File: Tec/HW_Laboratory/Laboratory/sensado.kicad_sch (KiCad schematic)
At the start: 3 parts, among them U5 INA3221, U6 INA3221, U7 LM75B

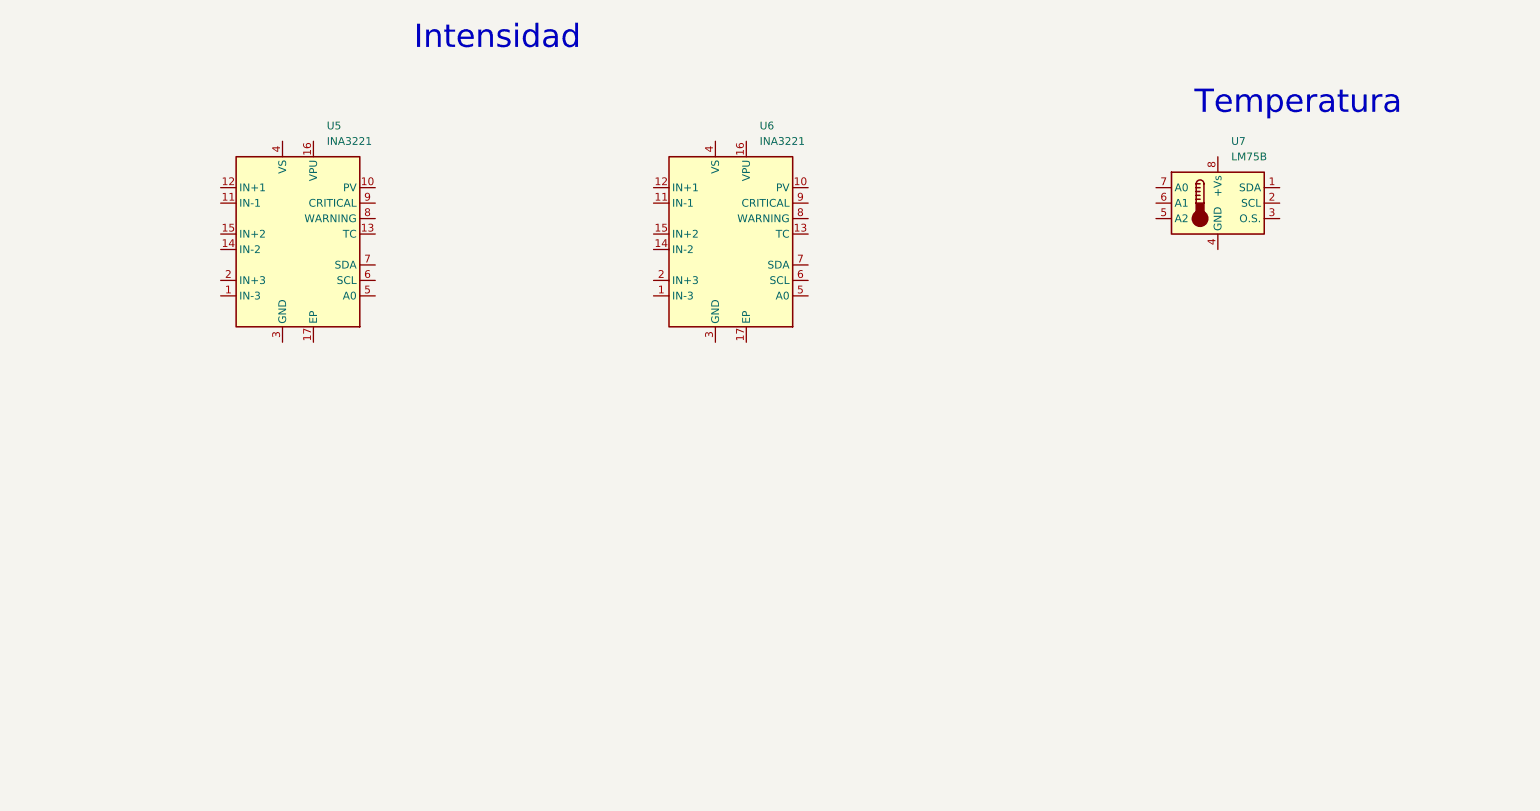
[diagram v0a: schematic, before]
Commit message: Schematics UPDATE
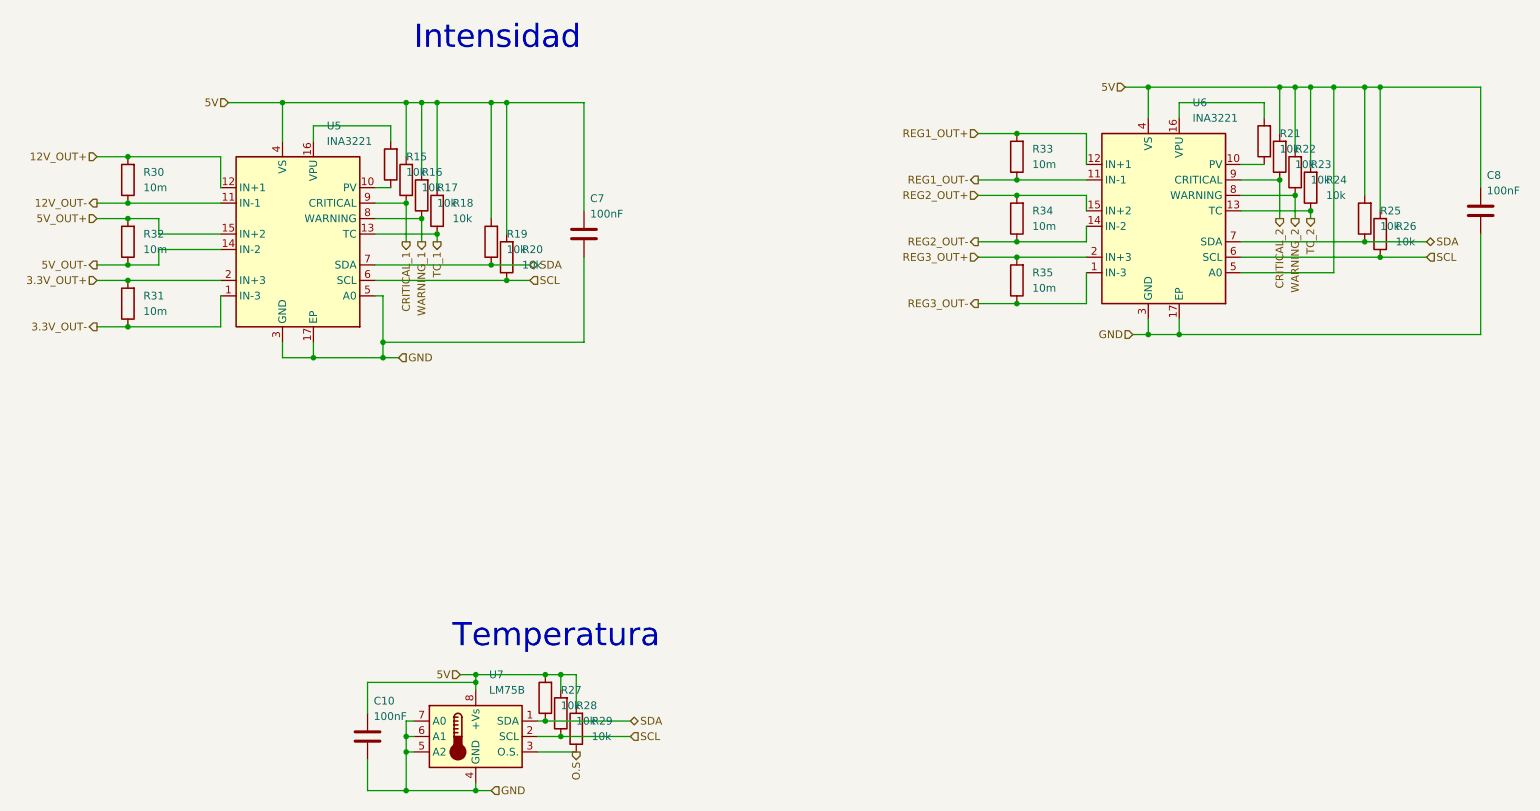
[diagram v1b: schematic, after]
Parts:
- added C10, C7, C8: 100nF, Capacitor_SMD:C_0603_1608Metric, symbol Device:C
- added R15, R16, R17, R18, R19, R20, R21, R22, R23, R24, R25, R26, R27, R28, R29: 10k, Resistor_SMD:R_0603_1608Metric, symbol Device:R
- added R30, R31, R32, R33, R34, R35: 10m, Resistor_SMD:R_2512_6332Metric, symbol Device:R
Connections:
- net 3.3V_OUT-: now reaches U5.1 (IN-3)
- net 3.3V_OUT-: now also R31.1
- net at U5.10 (PV): now also R15.1
- net 12V_OUT-: now reaches U5.11 (IN-1)
- net 12V_OUT-: now also R30.1
- net 12V_OUT+: now reaches U5.12 (IN+1)
- net 12V_OUT+: now also R30.2
- net TC_1: now reaches U5.13 (TC)
- net TC_1: now also R18.1
- net 5V_OUT-: now reaches U5.14 (IN-2)
- net 5V_OUT-: now also R32.1
- net 5V_OUT+: now reaches U5.15 (IN+2)
- net 5V_OUT+: now also R32.2
- net at U5.16 (VPU): now also R15.2
- net GND: now reaches U5.17 (EP)
- net GND: now also U5.3 (GND), U5.5 (A0), U6.17 (EP), U6.3 (GND), U7.4 (GND), U7.5 (A2), U7.6 (A1), U7.7 (A0), C10.2, C7.2, C8.2
- net 3.3V_OUT+: now reaches U5.2 (IN+3)
- net 3.3V_OUT+: now also R31.2
- net 5V: now reaches U5.4 (VS)
- net 5V: now also U6.4 (VS), U6.5 (A0), U7.8 (+Vs), C10.1, C7.1, C8.1, R16.2, R17.2, R18.2, R19.2, R20.2, R22.2, R23.2, R24.2, R25.2, R26.2, R27.2, R28.2, R29.2
- net SCL: now reaches U5.6 (SCL)
- net SCL: now also U6.6 (SCL), U7.2 (SCL), R20.1, R26.1, R28.1
- net SDA: now reaches U5.7 (SDA)
- net SDA: now also U6.7 (SDA), U7.1 (SDA), R19.1, R25.1, R27.1
- net WARNING_1: now reaches U5.8 (WARNING)
- net WARNING_1: now also R17.1
- net CRITICAL_1: now reaches U5.9 (CRITICAL)
- net CRITICAL_1: now also R16.1
- net O.S: now reaches U7.3 (O.S.)
- net O.S: now also R29.1
- net REG3_OUT-: now reaches U6.1 (IN-3)
- net REG3_OUT-: now also R35.1
- net at U6.10 (PV): now also R21.1
- net REG1_OUT-: now reaches U6.11 (IN-1)
- net REG1_OUT-: now also R33.1
- net REG1_OUT+: now reaches U6.12 (IN+1)
- net REG1_OUT+: now also R33.2
- net TC_2: now reaches U6.13 (TC)
- net TC_2: now also R24.1
- net REG2_OUT-: now reaches U6.14 (IN-2)
- net REG2_OUT-: now also R34.1
- net REG2_OUT+: now reaches U6.15 (IN+2)
- net REG2_OUT+: now also R34.2
- net at U6.16 (VPU): now also R21.2
- net REG3_OUT+: now reaches U6.2 (IN+3)
- net REG3_OUT+: now also R35.2
- net WARNING_2: now reaches U6.8 (WARNING)
- net WARNING_2: now also R23.1
- net CRITICAL_2: now reaches U6.9 (CRITICAL)
- net CRITICAL_2: now also R22.1
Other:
- moved on the sheet: U6, U7

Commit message: Schematics UPDATE
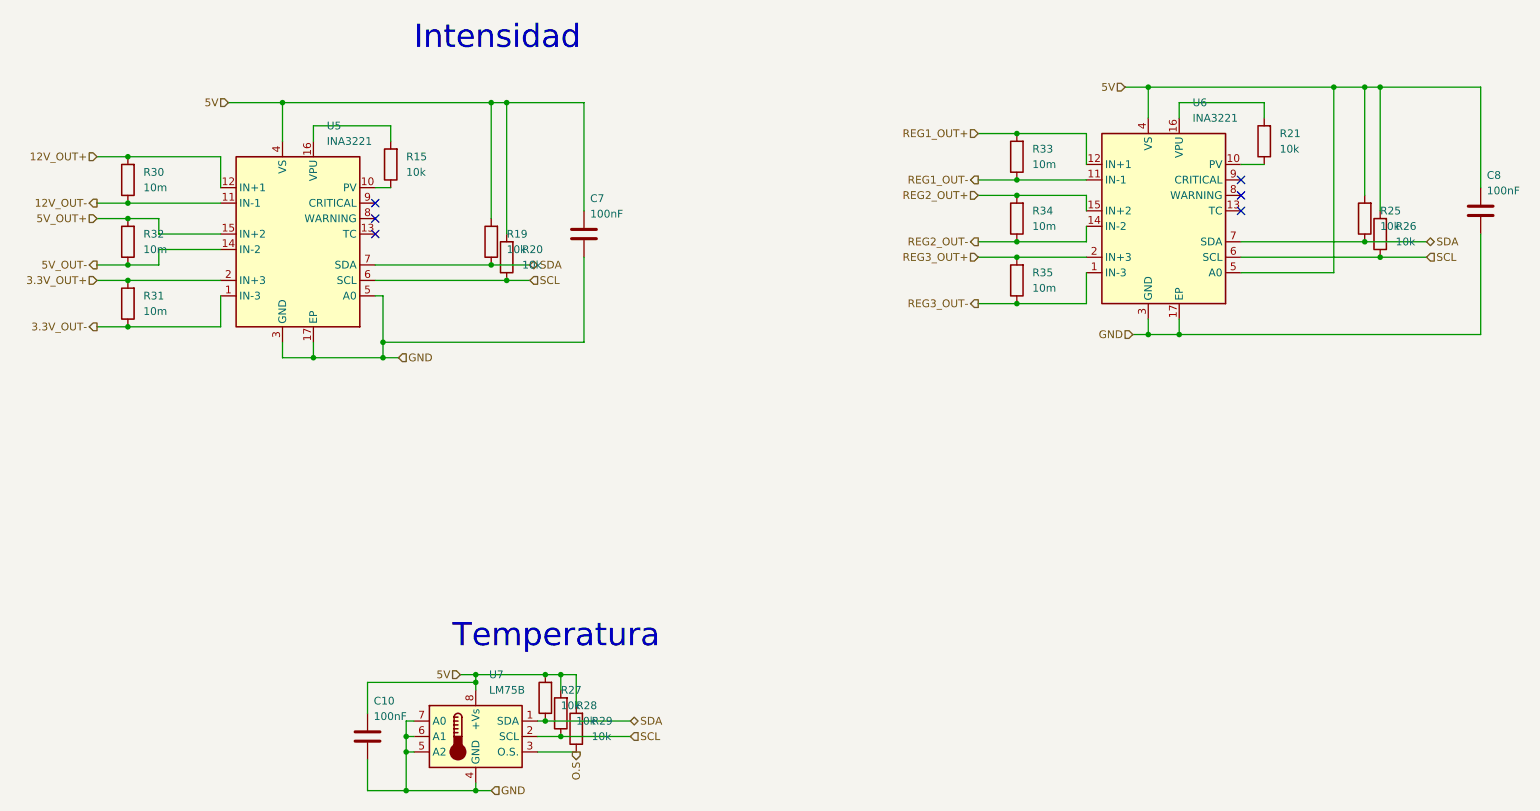
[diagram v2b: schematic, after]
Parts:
- removed R16, R17, R18, R22, R23, R24: 10k, Resistor_SMD:R_0603_1608Metric, symbol Device:R
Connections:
- net CRITICAL_1: no longer names the net of U5.9 (CRITICAL)
- net CRITICAL_2: no longer names the net of U6.9 (CRITICAL)
- net TC_1: no longer names the net of U5.13 (TC)
- net TC_2: no longer names the net of U6.13 (TC)
- net WARNING_1: no longer names the net of U5.8 (WARNING)
- net WARNING_2: no longer names the net of U6.8 (WARNING)
- no-connect marks 0 -> 6
